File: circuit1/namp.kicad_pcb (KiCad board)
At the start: 2 copper layers, 79 parts, among them J1 Screw_Terminal_01x08, J2 Screw_Terminal_01x04, J3 Screw_Terminal_01x04, U1 NRF52840-DONGLE, U2 MCP6004, U3 MCP6004, U4 MCP1501-33xSN, U5 MCP3564

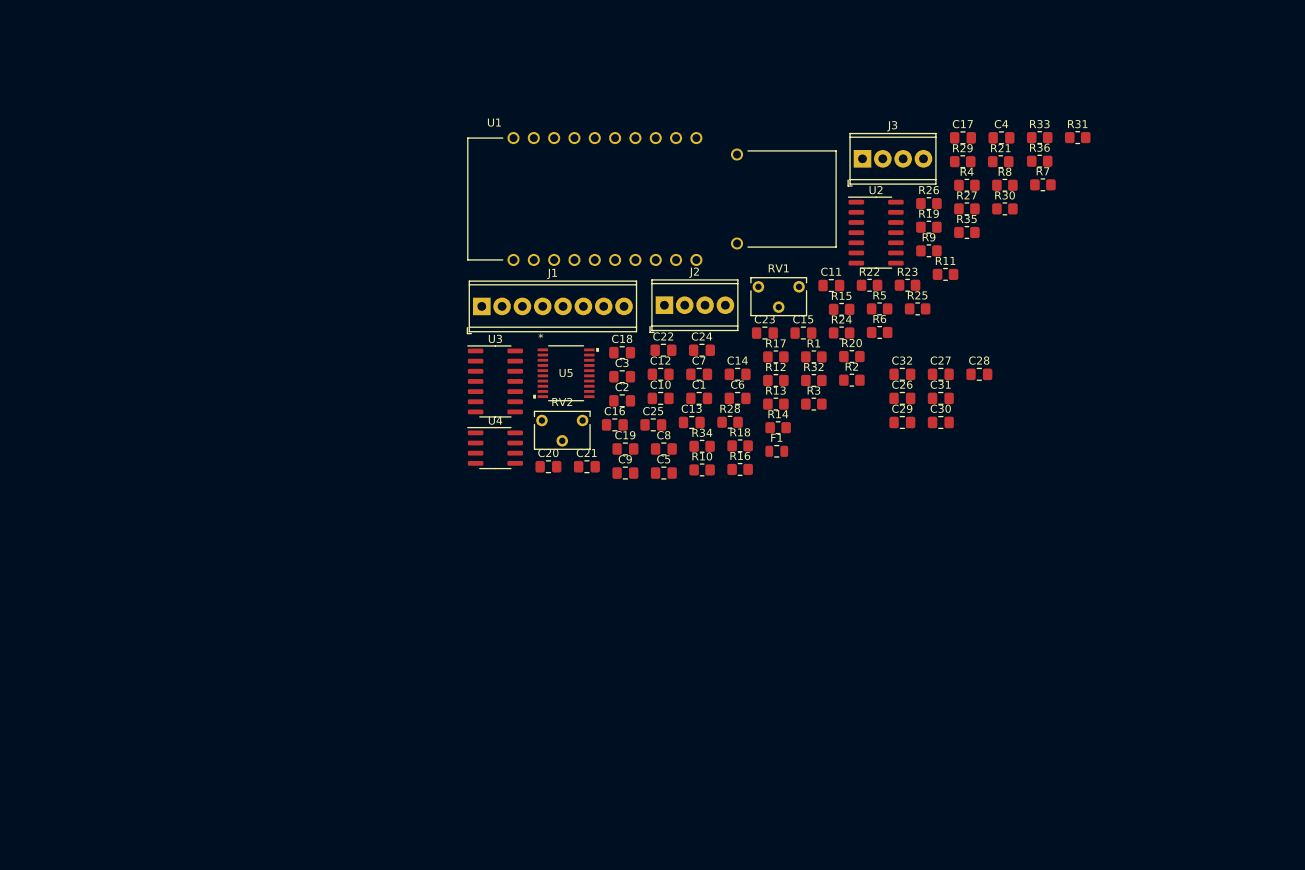
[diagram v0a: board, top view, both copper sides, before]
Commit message: update
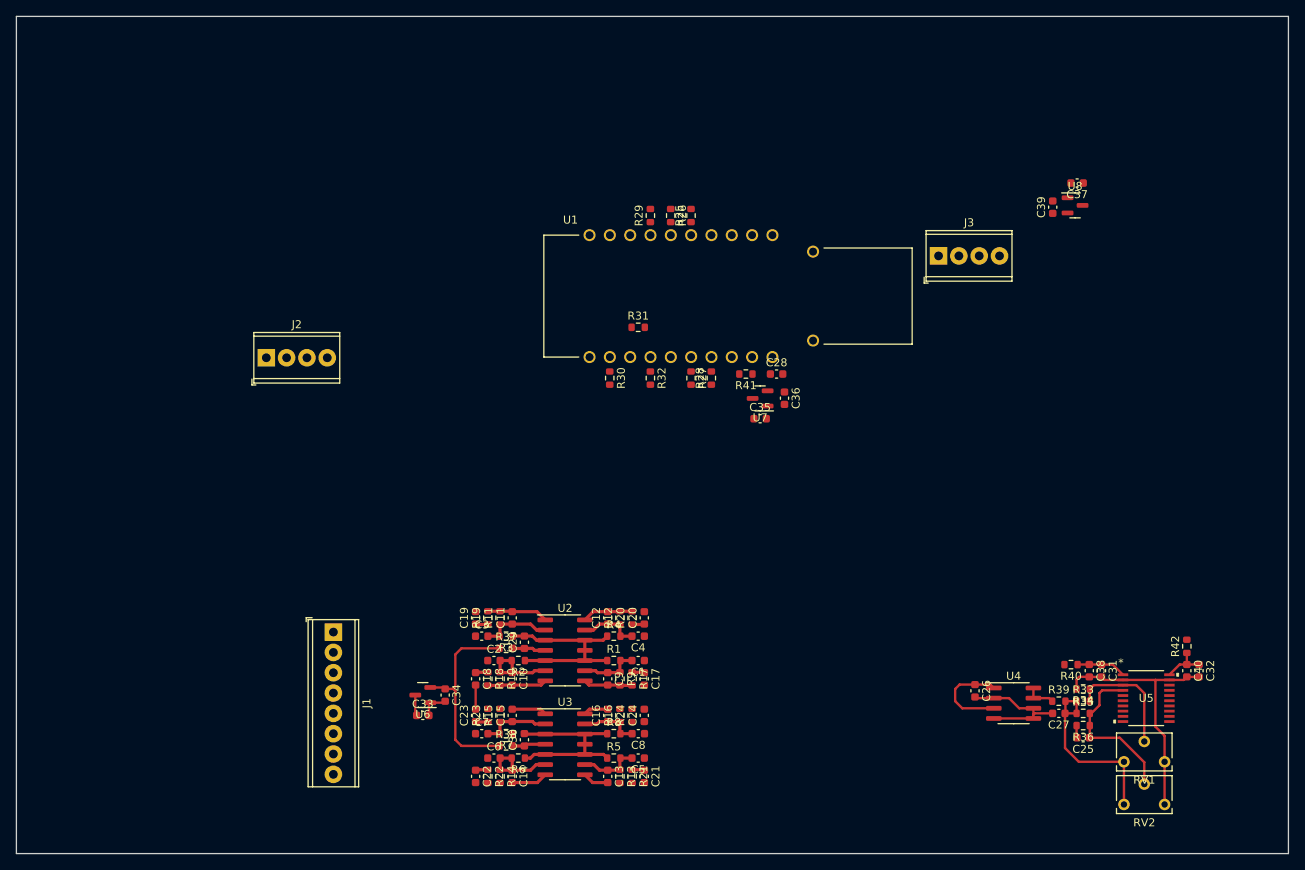
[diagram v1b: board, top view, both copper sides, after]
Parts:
- removed F1: 20mA, Fuse:Fuse_0805_2012Metric
- added C33: 1uF, Capacitor_SMD:C_0603_1608Metric, F.Cu at (112.8, 136.1)
- added C34: 1uF, Capacitor_SMD:C_0603_1608Metric, F.Cu at (115.6, 133.6)
- added C35: 1uF, Capacitor_SMD:C_0603_1608Metric, F.Cu at (154.9, 99.1)
- added C36: 1uF, Capacitor_SMD:C_0603_1608Metric, F.Cu at (158.0, 96.5)
- added C37: 1uF, Capacitor_SMD:C_0603_1608Metric, F.Cu at (194.6, 69.6)
- added C38: 10µF, Capacitor_SMD:C_0603_1608Metric, F.Cu at (196.1, 130.6)
- added C39: 1uF, Capacitor_SMD:C_0603_1608Metric, F.Cu at (191.5, 72.6)
- added C40: 10µF, Capacitor_SMD:C_0603_1608Metric, F.Cu at (208.3, 130.6)
- added R37: 10, Resistor_SMD:R_0603_1608Metric, F.Cu at (123.2, 127.8)
- added R38: 10, Resistor_SMD:R_0603_1608Metric, F.Cu at (123.2, 140.0)
- added R39: 100, Resistor_SMD:R_0603_1608Metric, F.Cu at (192.3, 134.4)
- added R40: 10, Resistor_SMD:R_0603_1608Metric, F.Cu at (193.8, 129.8)
- added R41: 10k, Resistor_SMD:R_0603_1608Metric, F.Cu at (153.2, 93.5)
- added R42: 10, Resistor_SMD:R_0603_1608Metric, F.Cu at (208.3, 127.5)
- added U6: MCP1754S-5002xCB, Package_TO_SOT_SMD:SOT-23, F.Cu at (112.8, 133.6)
- added U7: MCP1754S-5002xCB, Package_TO_SOT_SMD:SOT-23, F.Cu at (154.9, 96.5)
- added U8: MCP1754S-3302xCB, Package_TO_SOT_SMD:SOT-23, F.Cu at (194.3, 72.4)
- C1, C10, C11, C12, C13, C14, C15, C16, C17, C18, C19, C2, C20, C21, C22, C23, C24, C25, C28, C29, C3, C30, C4, C5, C6, C7, C8, C9: footprint Capacitor_SMD:C_0805_2012Metric_Pad1.18x1.45mm_HandSolder -> Capacitor_SMD:C_0603_1608Metric
- C26: value C -> 2.2µF; footprint Capacitor_SMD:C_0805_2012Metric_Pad1.18x1.45mm_HandSolder -> Capacitor_SMD:C_0603_1608Metric
- C27: value C -> 300pF; footprint Capacitor_SMD:C_0805_2012Metric_Pad1.18x1.45mm_HandSolder -> Capacitor_SMD:C_0603_1608Metric
- C31, C32: value C -> 0.1µF; footprint Capacitor_SMD:C_0805_2012Metric_Pad1.18x1.45mm_HandSolder -> Capacitor_SMD:C_0603_1608Metric
- R1, R10, R11, R12, R13, R14, R15, R16, R17, R18, R19, R2, R20, R21, R22, R23, R24, R25, R26, R27, R28, R29, R3, R30, R31, R32, R33, R34, R35, R36, R4, R5, R6, R7, R8, R9: footprint Resistor_SMD:R_0805_2012Metric_Pad1.20x1.40mm_HandSolder -> Resistor_SMD:R_0603_1608Metric
- moved R7 96.0 mm to (123.2, 138.4), turned to 180 degrees
- moved R21 89.6 mm to (138.9, 143.8), turned to -90 degrees
- moved R8 84.2 mm to (136.7, 138.4)
- moved U5 83.1 mm to (203.2, 134.0)
- moved RV2 83.0 mm to (200.4, 147.3), turned to 180 degrees
- moved C17 78.5 mm to (140.5, 131.6), turned to -90 degrees
- moved R22 77.7 mm to (120.9, 143.8), turned to -90 degrees
- moved C4 77.1 mm to (139.7, 126.2), turned to 180 degrees
- moved R23 75.1 mm to (120.9, 136.1), turned to 90 degrees
- moved R19 73.7 mm to (120.9, 124.0), turned to 90 degrees
- moved U4 72.2 mm to (186.6, 134.6)
- moved RV1 71.9 mm to (200.4, 141.9), turned to 180 degrees
- moved R4 71.6 mm to (136.7, 126.2)
- moved R36 70.8 mm to (195.3, 137.4), turned to 180 degrees
- moved R33 70.7 mm to (195.3, 134.4)
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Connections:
- net Net-(C25-Pad1) renamed REFIN+
- net Net-(U5-Pad3) renamed REFIN-
- C17 pad 2: GNDA -> GND
- C18 pad 2: GNDA -> GND
- C19 pad 2: GNDA -> GND
- C20 pad 2: GNDA -> GND
- C21 pad 2: GNDA -> GND
- C22 pad 2: GNDA -> GND
- C23 pad 2: GNDA -> GND
- C24 pad 2: GNDA -> GND
- C25 pad 2: GNDA -> GND
- C26 pad 1: +5V -> PWR_MAX16V
- C26 pad 2: GNDA -> GND
- C27 pad 1: Net-(U4-Pad7) -> ADC_VREF
- C27 pad 2: GNDA -> GND
- C28 pad 1: +5V -> Net-(C28-Pad1)
- C28 pad 2: GNDA -> GND
- C29 pad 1: ADC_AVDD -> Net-(C29-Pad1)
- C29 pad 2: GNDA -> GND
- C30 pad 1: ADC_AVDD -> Net-(C30-Pad1)
- C30 pad 2: GNDA -> GND
- C31 pad 1: ADC_AVDD -> AVDD
- C31 pad 2: GNDA -> GND
- C32 pad 1: V_REGOUT0 -> DVDD
- C32 pad 2: GNDA -> GND
- J2 pad 1: GNDA -> GND
- J2 pad 2: GNDA -> GND
- J2 pad 3: GNDA -> GND
- J2 pad 4: ADC_AVDD -> GND
- J3 pad 1: GNDA -> GND
- J3 pad 2: GNDA -> GND
- J3 pad 3: GNDA -> GND
- J3 pad 4: +5V -> PWR_MAX16V
- R1 pad 1: GNDA -> GND
- R2 pad 1: GNDA -> GND
- R3 pad 1: GNDA -> GND
- R33 pad 1: ADC_AVDD -> ADC_VREF
- R34 pad 2: GNDA -> GND
- R35 pad 1: ADC_AVDD -> ADC_VREF
- R36 pad 2: GNDA -> GND
- R4 pad 1: GNDA -> GND
- R5 pad 1: GNDA -> GND
- R6 pad 1: GNDA -> GND
- R7 pad 1: GNDA -> GND
- R8 pad 1: GNDA -> GND
- RV1 pad 1: ADC_AVDD -> ADC_VREF
- RV1 pad 3: GNDA -> GND
- RV2 pad 1: ADC_AVDD -> ADC_VREF
- RV2 pad 3: GNDA -> GND
- U1 pad G1: GNDA -> GND
- U1 pad G2: GNDA -> GND
- U1 pad G3: GNDA -> GND
- U1 pad VBUS: +5V -> Net-(C28-Pad1)
- U2 pad 10: GNDA -> GND
- U2 pad 11: GNDA -> GND
- U2 pad 12: GNDA -> GND
- U2 pad 3: GNDA -> GND
- U2 pad 4: ADC_AVDD -> Net-(C29-Pad1)
- U2 pad 5: GNDA -> GND
- U3 pad 10: GNDA -> GND
- U3 pad 11: GNDA -> GND
- U3 pad 12: GNDA -> GND
- U3 pad 3: GNDA -> GND
- U3 pad 4: ADC_AVDD -> Net-(C30-Pad1)
- U3 pad 5: GNDA -> GND
- U4 pad 1: +5V -> PWR_MAX16V
- U4 pad 2: GNDA -> GND
- U4 pad 3: +5V -> PWR_MAX16V
- U4 pad 4: GNDA -> GND
- U4 pad 5: GNDA -> GND
- U4 pad 6: GNDA -> GND
- U5 pad 1: ADC_AVDD -> AVDD
- U5 pad 19: GNDA -> GND
- U5 pad 2: GNDA -> GND
- U5 pad 20: V_REGOUT0 -> DVDD
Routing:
- net GND: track 0.00 -> 106.4 mm
- net Net-(C34-Pad1): track 0.00 -> 25.5 mm
- net ADC_VREF: track 0.00 -> 23.7 mm
- net REFIN+: track 0.00 -> 20.2 mm
- net REFIN-: track 0.00 -> 15.0 mm
- net PWR_MAX16V: track 0.00 -> 14.6 mm
- net Net-(C14-Pad1): track 0.00 -> 10.4 mm
- net Net-(C10-Pad1): track 0.00 -> 10.2 mm
- net Net-(C11-Pad1): track 0.00 -> 8.92 mm
- net Net-(C15-Pad1): track 0.00 -> 8.74 mm
- net Net-(C12-Pad1): track 0.00 -> 7.65 mm
- net Net-(C13-Pad1): track 0.00 -> 7.63 mm
- net Net-(C11-Pad2): track 0.00 -> 7.62 mm
- net Net-(C16-Pad1): track 0.00 -> 7.47 mm
- net Net-(C1-Pad2): track 0.00 -> 7.45 mm
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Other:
- board outline added: 159 x 104.6 mm
